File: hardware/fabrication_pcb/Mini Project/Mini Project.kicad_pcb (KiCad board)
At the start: 2 copper layers, 10 parts, among them SW1 SW_Push, SW2 SW_Push, SW3 SW_Push, SW4 SW_Push

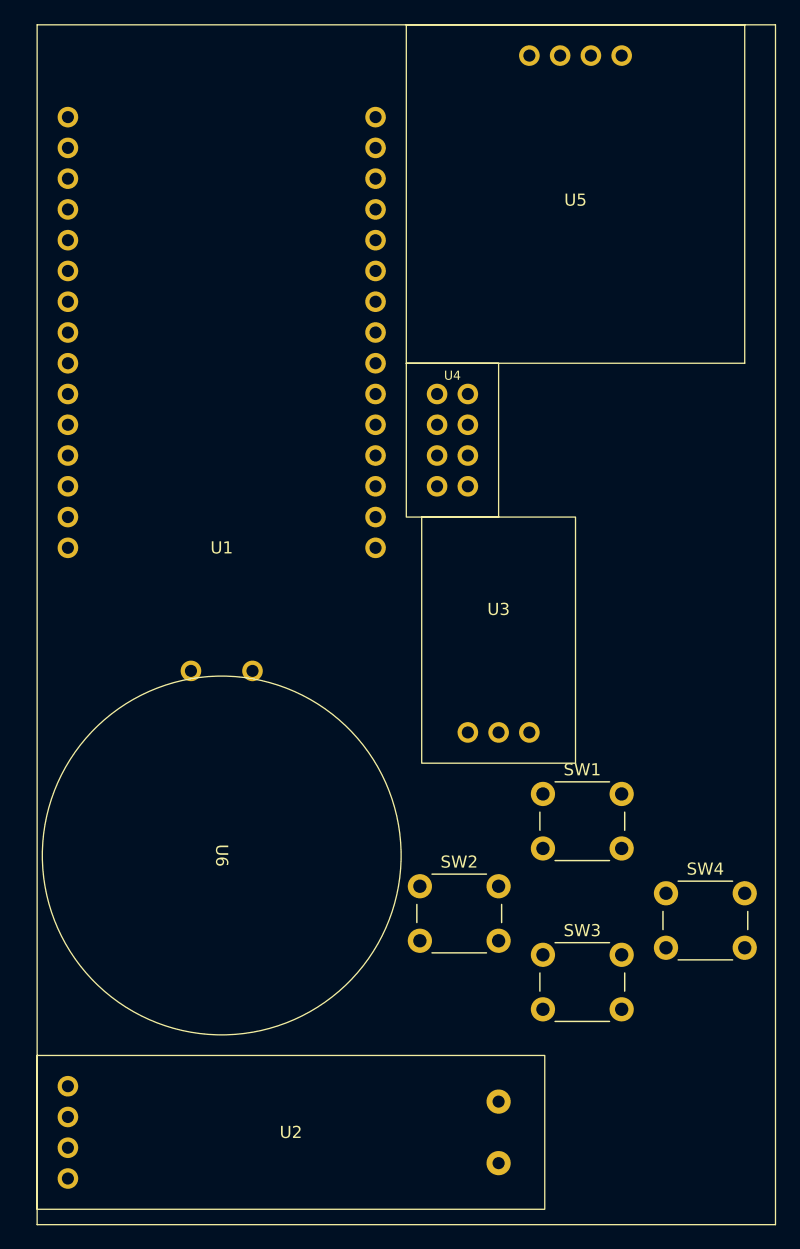
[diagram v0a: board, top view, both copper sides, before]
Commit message: feat: very bad basic routing
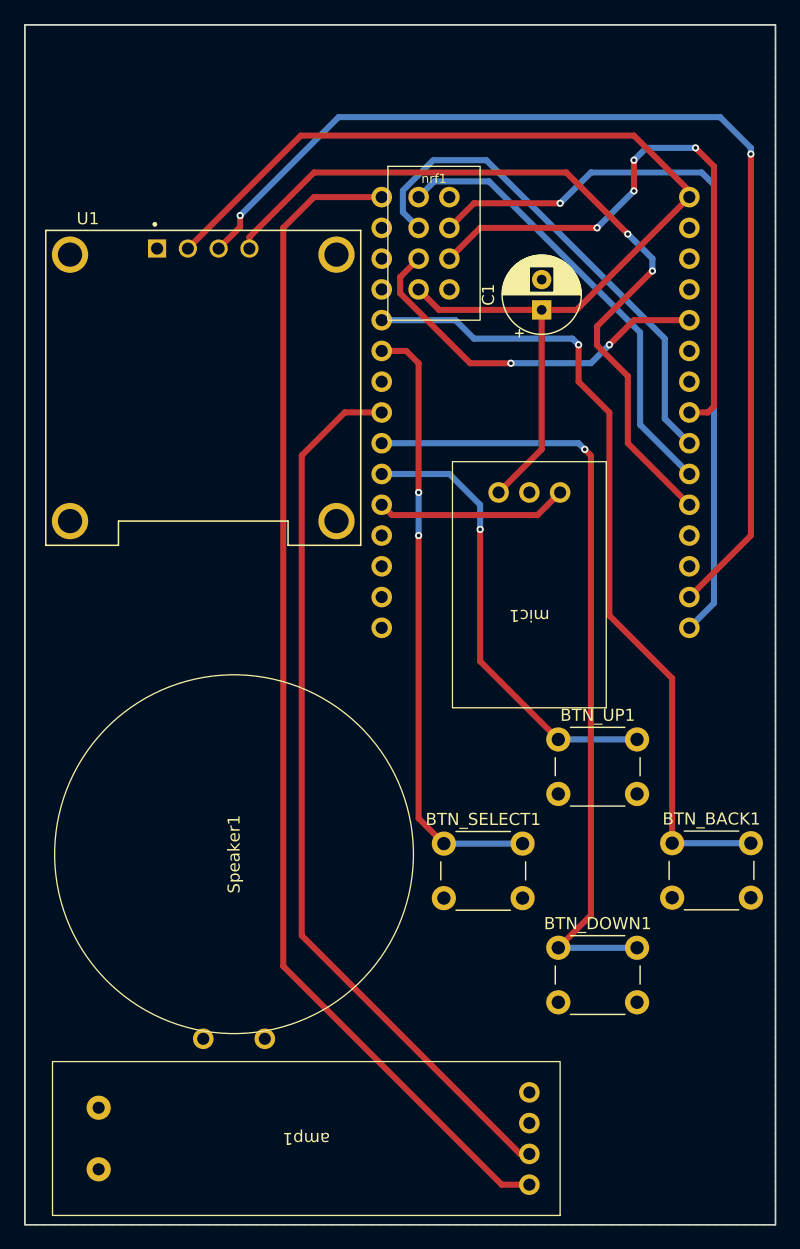
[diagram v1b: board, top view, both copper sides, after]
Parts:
- removed SW1, SW2, SW3, SW4: SW_Push, Button_Switch_THT:SW_PUSH_6mm
- removed U2: ~, MyFootprints:LM386_MODULE
- removed U3: ~, MyFootprints:MAX4466_MODULE
- removed U4: ~, MyFootprints:NRF24L01_PA_LNA
- removed U5: ~, MyFootprints:OLED_128x64_I2C
- removed U6: ~, MyFootprints:0.25W_8OHM_SPEAKER
- added BTN_BACK1: SW_Push, Button_Switch_THT:SW_PUSH_6mm, F.Cu at (176.9, 110.7)
- added BTN_DOWN1: SW_Push, Button_Switch_THT:SW_PUSH_6mm, F.Cu at (167.5, 119.4)
- added BTN_SELECT1: SW_Push, Button_Switch_THT:SW_PUSH_6mm, F.Cu at (158.0, 110.8)
- added BTN_UP1: SW_Push, Button_Switch_THT:SW_PUSH_6mm, F.Cu at (167.5, 102.2)
- added C1: 47nF, Capacitor_THT:CP_Radial_D6.3mm_P2.50mm, F.Cu at (166.1, 66.7)
- added Speaker1: ~, MyFootprints:0.25W_8OHM_SPEAKER, F.Cu at (138.2, 126.9)
- added amp1: ~, MyFootprints:LM386_MODULE, F.Cu at (165.1, 138.9)
- added esp32: ~, MyFootprints:ESP32_DevKit_V1_30pin, B.Cu at (178.3, 57.4)
- added mic1: ~, MyFootprints:MAX4466_MODULE, F.Cu at (167.6, 81.8)
- added nrf1: ~, MyFootprints:NRF24L01_PA_LNA, F.Cu at (156.0, 65.0)
- U1: value ~ -> DM-OLED096-636; footprint MyFootprints:ESP32_DevKit_V1_30pin -> SH1106:MODULE_DM-OLED096-636
- moved U1 25.0 mm to (138.2, 73.2)
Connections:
- U1 pad 1: unconnected-(U1-3V3-Pad1) -> GND
- U1 pad 2: unconnected-(U1-GND-Pad2) -> VCC
- U1 pad 3: unconnected-(U1-D15-Pad3) -> SCL
- U1 pad 4: unconnected-(U1-D2-Pad4) -> SDA
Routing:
- net amp_V: track 0.00 -> 97.9 mm
- net VCC: track 0.00 -> 91.1 mm
- net SCL: track 0.00 -> 89.2 mm, vias 0 -> 2
- net dac_out: track 0.00 -> 74.0 mm
- net Net-(esp32-D14): track 0.00 -> 67.9 mm, vias 0 -> 1
- net Net-(esp32-D33): track 0.00 -> 65.9 mm, vias 0 -> 1
- net SDA: track 0.00 -> 64.7 mm, vias 0 -> 2
- net MOSI: track 0.00 -> 61.6 mm, vias 0 -> 1
- net Net-(esp32-D27): track 0.00 -> 50.5 mm, vias 0 -> 2
- net CSN: track 0.00 -> 49.8 mm, vias 0 -> 4
- net SCK: track 0.00 -> 41.9 mm
- net Net-(esp32-D32): track 0.00 -> 37.7 mm, vias 0 -> 1
- net MISO: track 0.00 -> 37.4 mm
- net CE: track 0.00 -> 31.2 mm, vias 0 -> 2
- net adc_inp: track 0.00 -> 15.9 mm
- added copper zone on B.Cu, net GND
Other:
- board outline added: 62 x 99.1 mm
